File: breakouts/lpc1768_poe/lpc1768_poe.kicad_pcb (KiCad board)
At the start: 2 copper layers, 113 parts, among them J1 extra, J2 usb, J3 jtag/uart, J4 RC02535, Q1 DMP3099L-7, SW1 btn, U1 LD39020ATPU33R, U2 LPC1768FET100, U3 Si3402-C, U4 RTL8201F-VB-CG, Y1 12MHz, Y2 25MHz

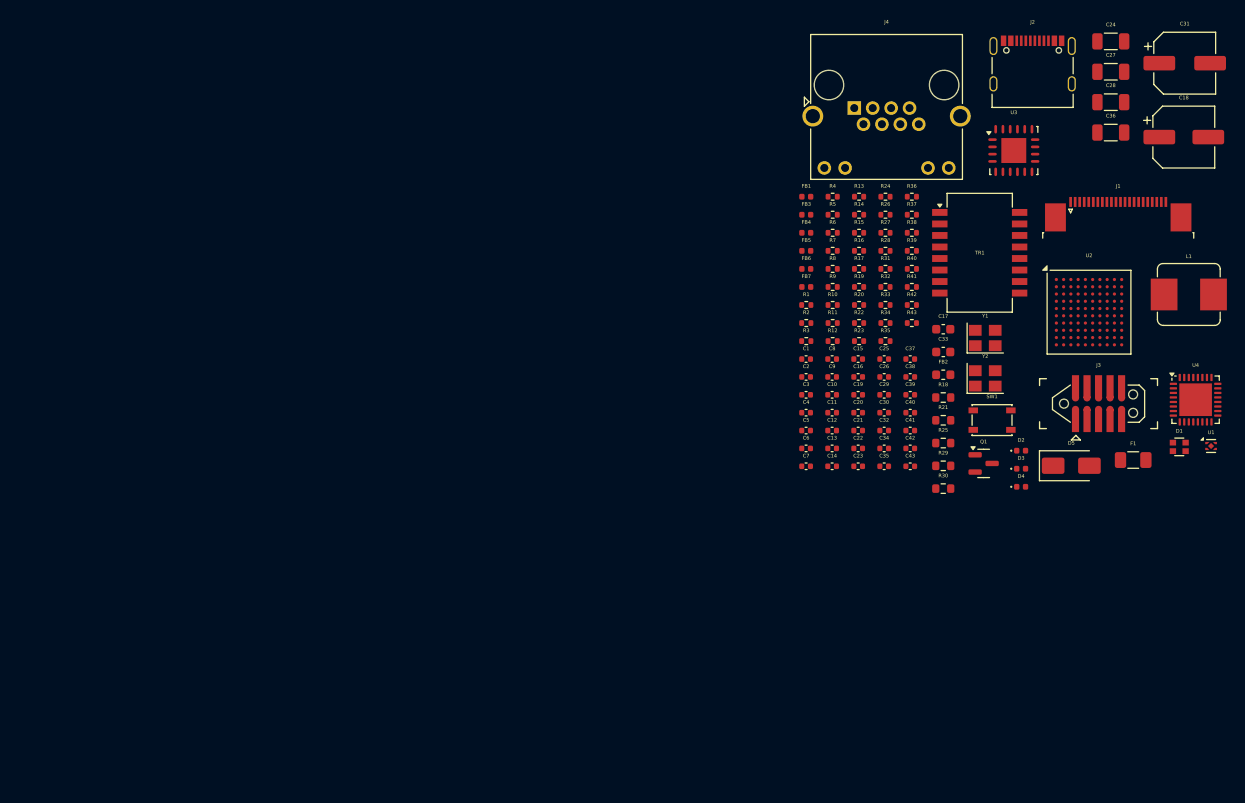
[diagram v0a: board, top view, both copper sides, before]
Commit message: finish lpc1768_poe layout
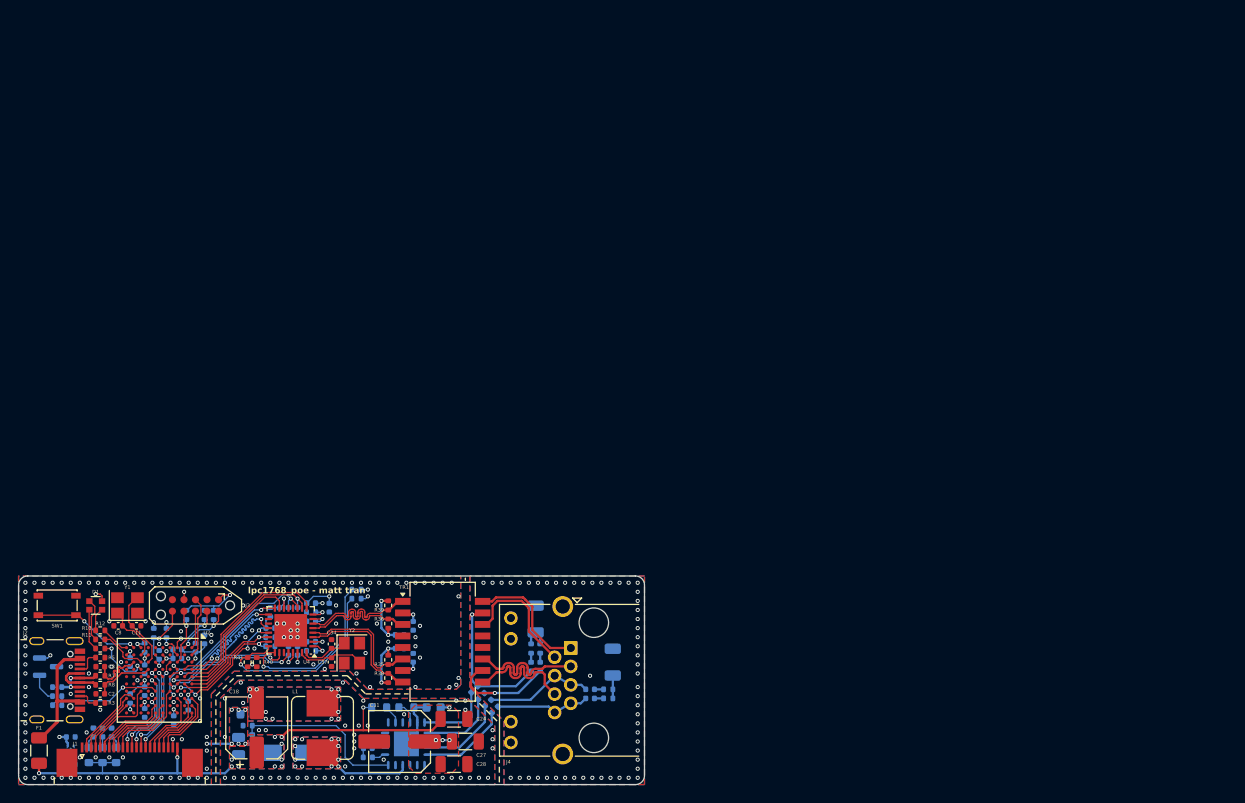
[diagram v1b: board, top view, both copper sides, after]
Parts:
- added C44: 1n, Capacitor_SMD:C_1206_3216Metric, B.Cu at (200.0, 98.0)
- added R44: 0, Resistor_SMD:R_0402_1005Metric, B.Cu at (138.8, 102.8)
- C1, C10, C12, C13, C14, C15, C16, C19, C20, C21, C22, C23, C25, C26, C29, C30, C32, C33, C35, C36, C38, C39, C4, C40, C41, C42, C43, C5, C6, C7, C9, D2, D3, D4, D5, FB1, FB2, FB3, FB4, FB5, FB6, FB7, Q1, R1, R13, R14, R15, R16, R17, R18, R19, R2, R20, R21, R22, R23, R24, R25, R26, R27, R28, R29, R30, R31, R32, R33, R34, R37, R4, R42, R43, R6, R9, U1, U3: moved to B.Cu
- C17: footprint Capacitor_SMD:C_0603_1608Metric -> Capacitor_SMD:C_0805_2012Metric; moved to B.Cu
- J3: footprint extraparts:TC2050+Header -> Connector:Tag-Connect_TC2050-IDC-NL_2x05_P1.27mm_Vertical
- moved U1 130.1 mm to (140.2, 107.8), turned to -90 degrees
- moved J2 127.2 mm to (138.8, 100.0), turned to -90 degrees
- moved F1 124.8 mm to (136.8, 107.8), turned to -90 degrees
- moved J1 124.5 mm to (146.8, 108.8)
- moved C18 121.2 mm to (160.8, 105.2), turned to 90 degrees
- moved D1 120.7 mm to (143.0, 91.8), turned to 180 degrees
- moved C31 114.4 mm to (176.5, 106.8), turned to 180 degrees
- moved U2 110.2 mm to (150.0, 100.0), turned to -90 degrees
- moved D2 106.9 mm to (142.8, 105.8), turned to -90 degrees
- moved L1 106.8 mm to (168.0, 105.2), turned to -90 degrees
- moved Q1 105.5 mm to (137.8, 98.5)
- moved D3 105.4 mm to (143.8, 105.8), turned to -90 degrees
- moved SW1 105.1 mm to (138.8, 91.8), turned to 180 degrees
- moved C24 104.0 mm to (182.5, 104.2)
- moved D4 103.9 mm to (144.8, 105.8), turned to -90 degrees
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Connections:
- C19 pad 1: Net-(U4-PHYRSTB) -> /phy_rst
- FB4 pad 2: /eth_tx_cm -> Net-(C41-Pad1)
- FB5 pad 2: Net-(C38-Pad1) -> /eth_rx_cm
- FB6 pad 2: /eth_rx_cm -> Net-(C38-Pad1)
- FB7 pad 2: Net-(C41-Pad1) -> /eth_tx_cm
- J1 pad 10: /p0.15 -> /p0.5
- J1 pad 11: /p0.11 -> /p0.16
- J1 pad 12: /p0.10 -> /p0.18
- J1 pad 13: /p0.9 -> /p1.31
- J1 pad 14: /p0.8 -> /p0.23
- J1 pad 15: /p0.7 -> /p0.26
- J1 pad 16: /p0.6 -> /p0.8
- J1 pad 17: /p0.5 -> /p0.6
- J1 pad 18: /p0.4 -> /p0.9
- J1 pad 19: /p0.1 -> /p0.7
- J1 pad 2: /p2.8 -> /p0.1
- J1 pad 20: /p0.0 -> /p0.4
- J1 pad 3: /p2.7 -> /p0.0
- J1 pad 4: /p1.31 -> /p0.11
- J1 pad 5: /p0.26 -> /p0.10
- J1 pad 6: /p0.23 -> /p0.17
- J1 pad 7: /p0.18 -> /p0.15
- J1 pad 8: /p0.17 -> /p2.7
- J1 pad 9: /p0.16 -> /p2.8
- J3 pad 10: /nrst -> /jtms
- J3 pad 2: /jtms -> GND
- J3 pad 3: GND -> /dbg_rx
- J3 pad 4: /jtck -> /dbg_tx
- J3 pad 5: /dbg_rx -> GND
- J3 pad 6: /jtdo -> /nrst
- J3 pad 7: /dbg_tx -> /jtdi
- J3 pad 8: /jtdi -> /jtdo
- J3 pad 9: GND -> /jtck
- R27 pad 2: Net-(U4-PHYRSTB) -> /phy_rst
- R34 pad 2: Net-(C36-Pad1) -> Net-(C44-Pad1)
- R35 pad 2: /eth_rx+ -> /eth_tx-
- R36 pad 1: /eth_tx- -> /eth_rx+
- R37 pad 2: Net-(C36-Pad1) -> Net-(C44-Pad1)
- R38 pad 2: /eth_rx- -> /eth_tx+
- R39 pad 1: /eth_tx+ -> /eth_rx-
- R42 pad 2: /eth_led0 -> /eth_led1
- R43 pad 2: /eth_led1 -> /eth_led0
- TR1 pad 1: /eth_tx+ -> /eth_rx-
- TR1 pad 3: /eth_tx- -> /eth_rx+
- TR1 pad 6: /eth_rx+ -> /eth_tx-
- TR1 pad 8: /eth_rx- -> /eth_tx+
- U2 pad C7: unconnected-(U2-P4[28]-PadC7) -> /phy_rst
- U2 pad H3: /led_g -> /led_b
- U2 pad H4: /led_r -> /led_g
- U2 pad K1: /led_b -> /led_r
- U4 pad 21: Net-(U4-PHYRSTB) -> /phy_rst
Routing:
- net +5V: track 0.00 -> 57.9 mm, vias 0 -> 16
- net +3V3: track 0.00 -> 43.2 mm, vias 0 -> 16
- net Net-(J4-Pad12): track 0.00 -> 31.3 mm, vias 0 -> 1
- net GND: track 0.00 -> 23.1 mm, vias 0 -> 160
- net /eth_led0: track 0.00 -> 22.5 mm, vias 0 -> 1
- net /rmii_int: track 0.00 -> 22.3 mm, vias 0 -> 2
- net /rmii_rx0: track 0.00 -> 20.0 mm
- net Net-(J4-Pad10): track 0.00 -> 19.8 mm, vias 0 -> 1
- net /rmii_rx1: track 0.00 -> 19.5 mm, vias 0 -> 1
- net /eth_led1: track 0.00 -> 19.4 mm, vias 0 -> 1
- net Net-(U3-FB): track 0.00 -> 19.3 mm
- net /rmii_ref_clk: track 0.00 -> 17.8 mm
- net /phy_rst: track 0.00 -> 16.8 mm, vias 0 -> 4
- net /eth_tx_cm: track 0.00 -> 16.0 mm, vias 0 -> 1
- net /rmii_rx_er: track 0.00 -> 15.4 mm, vias 0 -> 2
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- added copper zone on In2.Cu, net +3V3
- added copper zone on B.Cu, net +5V
- added copper zone on F.Cu, net +5V
- added copper zone on In1.Cu, net +5V
- added copper zone on In2.Cu, net +5V
- added copper zone on B.Cu, net GND
- added copper zone on F.Cu, net GND
- added copper zone on In1.Cu, net GND
- added copper zone on In2.Cu, net GND
- added copper zone on B.Cu, net GND_BS
- added copper zone on F.Cu, net GND_BS
- added copper zone on In1.Cu, net GND_BS
- added copper zone on In2.Cu, net GND_BS
- added copper zone on B.Cu, net GND_RTN
- added copper zone on F.Cu, net GND_RTN
- added copper zone on In1.Cu, net GND_RTN
- added copper zone on In2.Cu, net GND_RTN
- added copper zone on B.Cu, net Net-(C18-Pad2)
- added copper zone on F.Cu, net Net-(C18-Pad2)
- added copper zone on In1.Cu, net Net-(C18-Pad2)
- added copper zone on In2.Cu, net Net-(C18-Pad2)
- added copper zone on B.Cu, net Net-(D5-A)
- added copper zone on F.Cu, net Net-(D5-A)
- added copper zone on In1.Cu, net Net-(D5-A)
- added copper zone on In2.Cu, net Net-(D5-A)
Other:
- board outline added: 69 x 23 mm
- copper layers 2 -> 4
- board text added: "lpc1768_poe - matt tran"
